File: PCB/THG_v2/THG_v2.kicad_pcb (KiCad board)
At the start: 2 copper layers, 50 x 69.5 mm, 11 parts, among them J1 AM2315_Conn, J2 LCD_conn, J3 RTC_Conn, J4 SD_card_conn, J5 AC_in_terminal, U1 mini_esp32

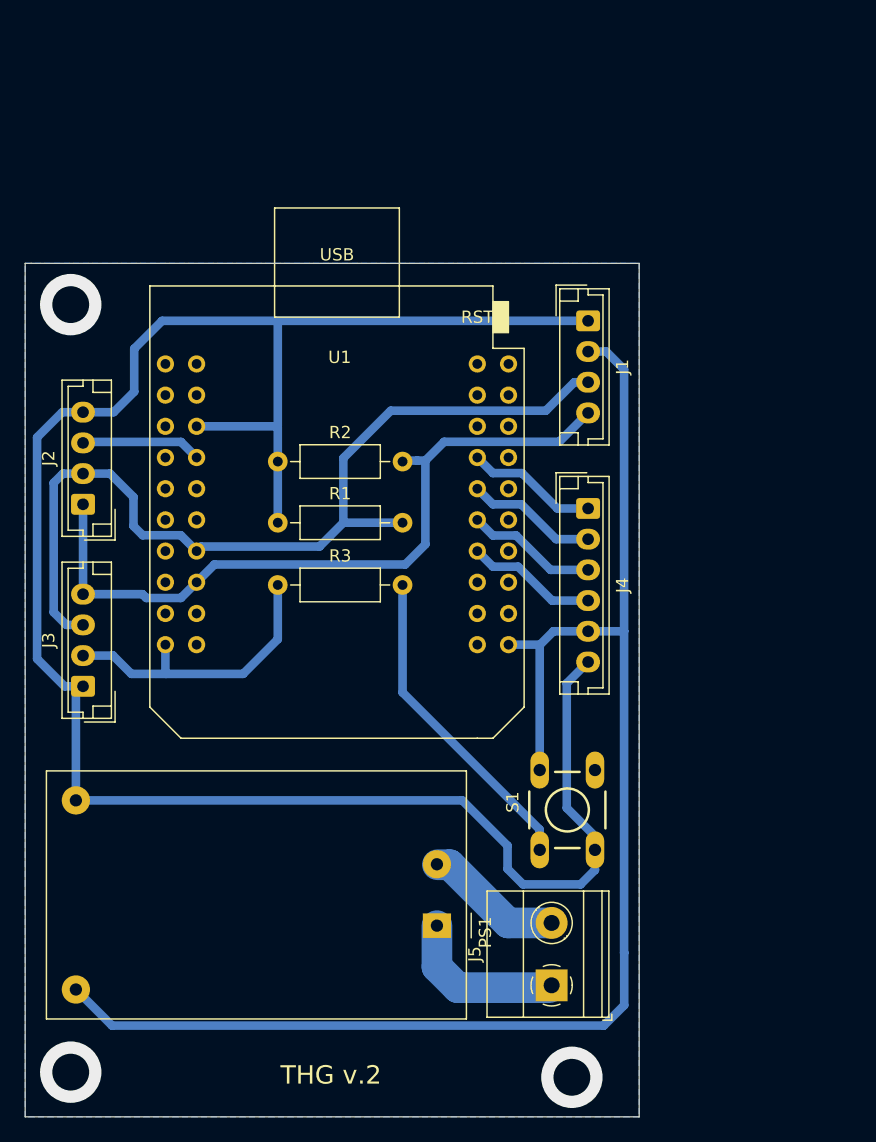
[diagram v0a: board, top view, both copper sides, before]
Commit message: fix cordinate
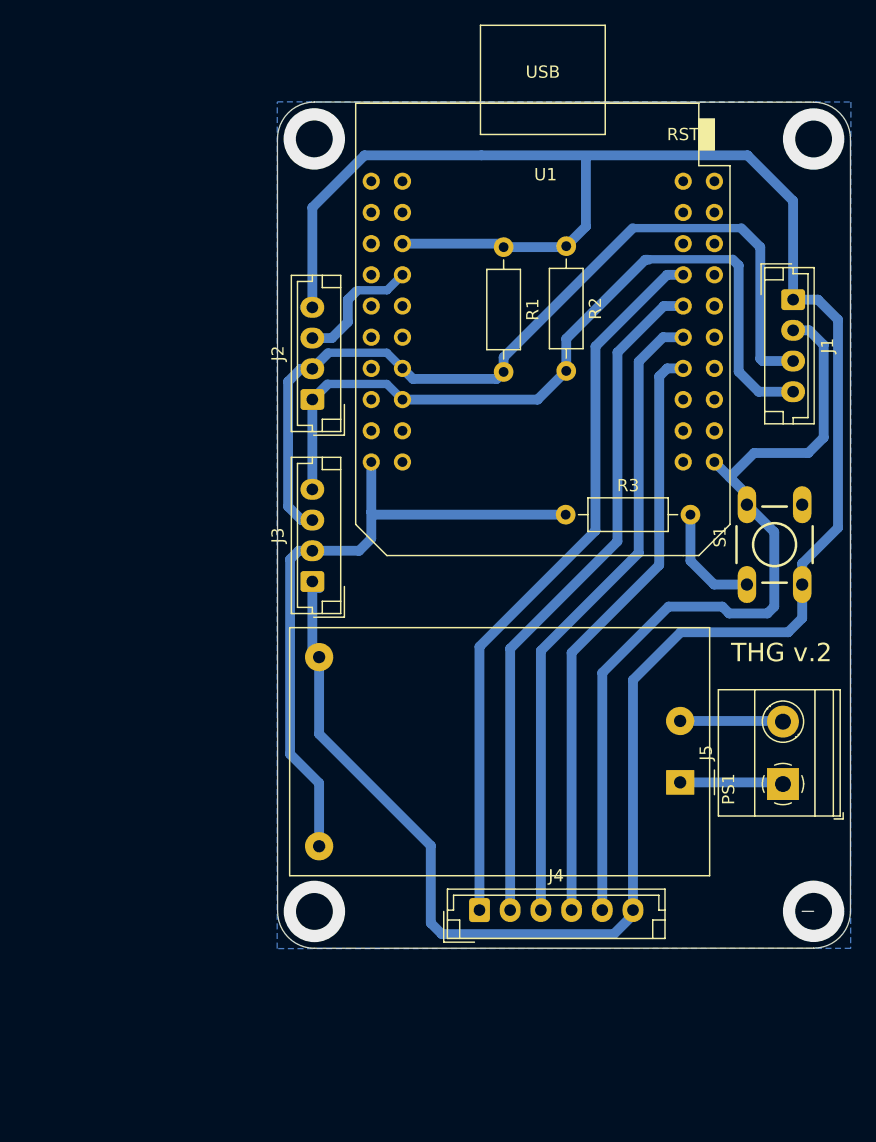
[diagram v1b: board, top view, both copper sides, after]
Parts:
- moved J4 33.9 mm to (155.5, 115.2), turned to 0 degrees
- moved R2 29.3 mm to (162.6, 61.1), turned to -90 degrees
- moved R1 29.0 mm to (157.5, 61.2), turned to -90 degrees
- moved S1 27.4 mm to (179.5, 85.4)
- moved J5 25.0 mm to (180.2, 104.9)
- moved R3 24.1 mm to (162.5, 83.0)
- moved PS1 23.0 mm to (171.8, 104.8)
- moved U1 22.4 mm to (160.7, 67.2)
- moved J2 20.5 mm to (141.9, 73.6)
- moved J3 20.5 mm to (141.9, 88.4)
- moved J1 16.8 mm to (181.0, 65.5)
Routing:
- net GPIO5: track 10.7 -> 59.4 mm
- net GPIO23: track 10.7 -> 56.0 mm
- net GPIO19: track 10.7 -> 52.4 mm
- net GPIO18: track 10.7 -> 48.6 mm
- net +5V: track 171.6 -> 195.7 mm
- net GND: track 156.2 -> 134.3 mm
- net Net-(S1-Pad1): track 26.2 -> 9.16 mm
- net Net-(J5-Pad1): track 13.5 -> 8.43 mm
- net SDA: track 74.8 -> 71.2 mm
- net Net-(J5-Pad2): track 11.3 -> 8.40 mm
- net SCL: track 60.7 -> 63.3 mm
- net (no net): vias 3 -> 4
- added copper zone on B.Cu, net +5V
- removed copper zone on B.Cu, net GND
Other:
- board size 50 x 69.5 mm -> 46.7 x 68.9 mm

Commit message: rev
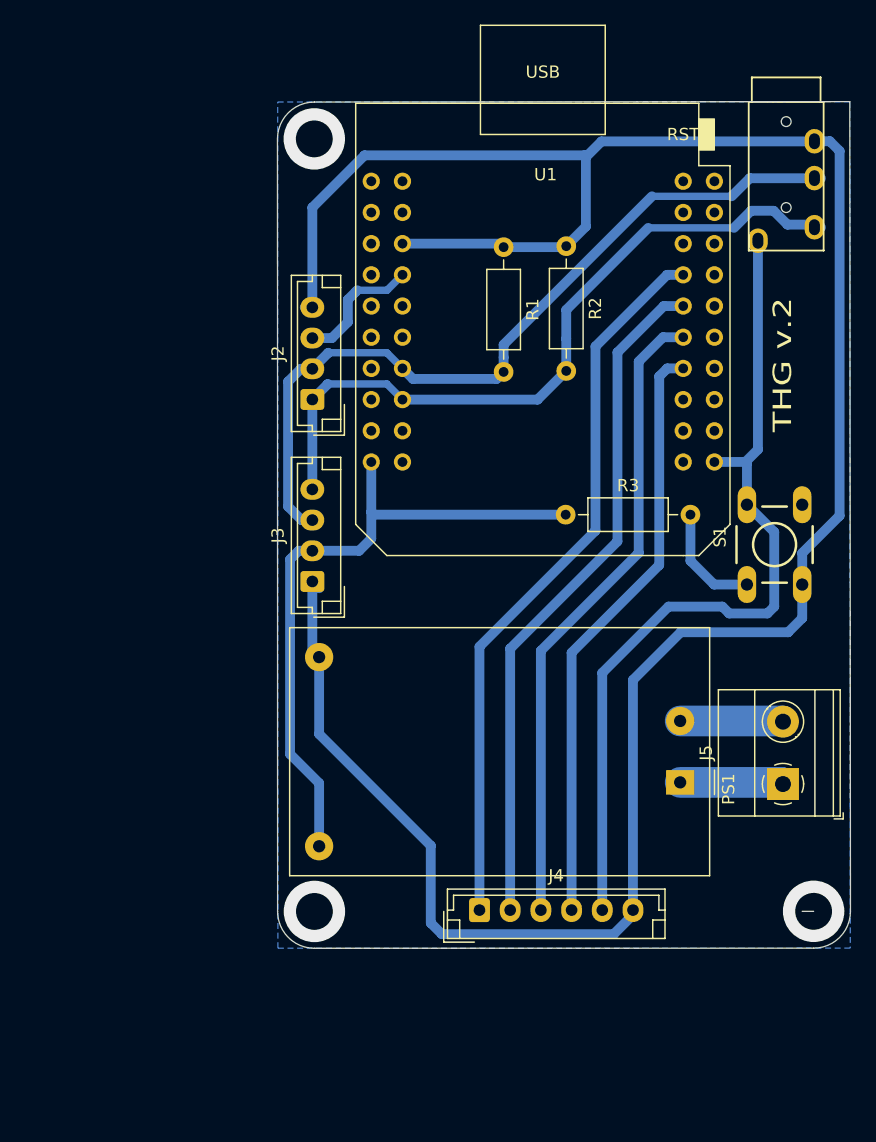
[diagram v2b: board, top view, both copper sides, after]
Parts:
- J1: value AM2315_Conn -> AM2315_Jack; footprint Connector_JST:JST_EH_B4B-EH-A_1x04_P2.50mm_Vertical -> Lib_Kicad:TRRS-PJ-320A
- moved J1 16.1 mm to (180.5, 49.4), turned to 0 degrees
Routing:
- net SDA: track 71.2 -> 65.9 mm
- net +5V: track 195.7 -> 200.8 mm
- net SCL: track 63.3 -> 59.6 mm
- net (no net): vias 4 -> 3
- added copper zone on B.Cu, net GND
- removed copper zone on B.Cu, net +5V
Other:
- outline, holes or cut-outs redrawn
